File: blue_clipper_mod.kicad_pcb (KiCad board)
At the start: 2 copper layers, 68.6 x 50.8 mm, 23 parts, among them J1 AudioJack3, J2 AudioJack2, SW1 SW_Rotary_1x4_MP, SW2 SW_Rotary_1x4_MP, U1 RC4558

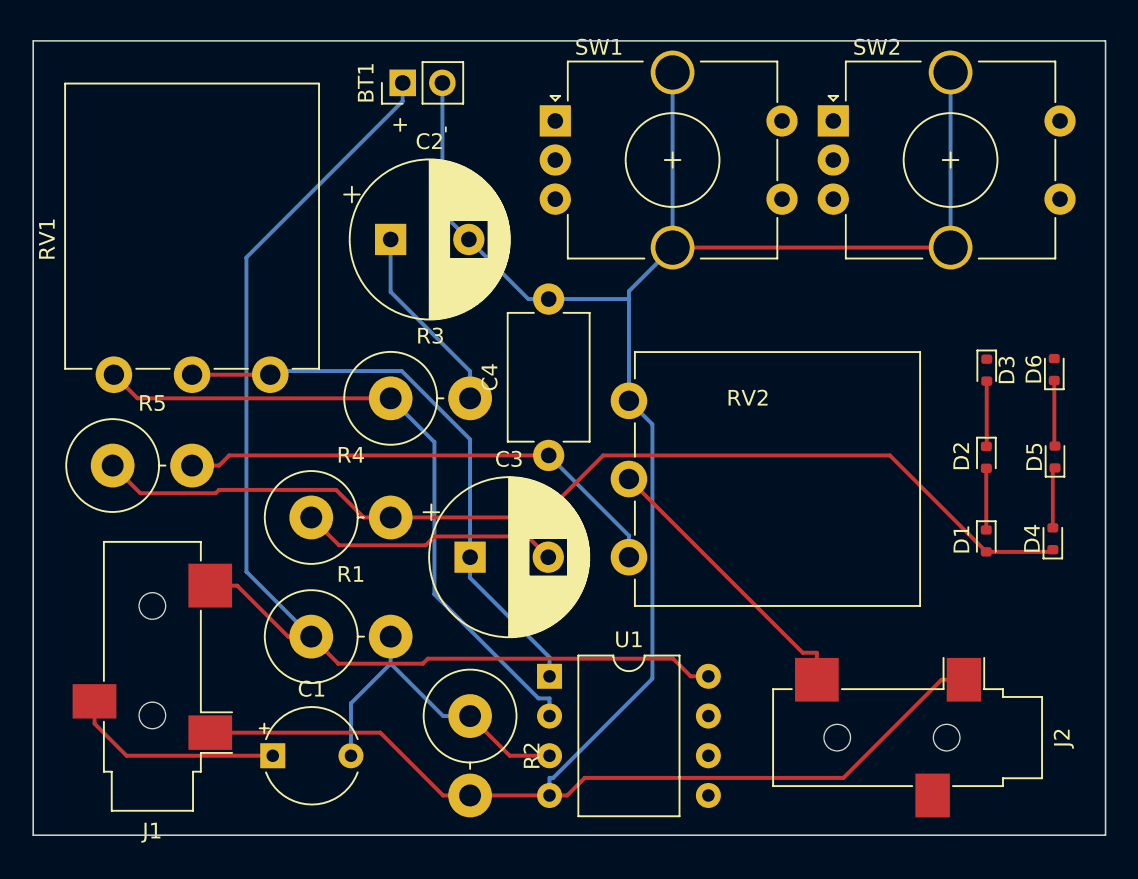
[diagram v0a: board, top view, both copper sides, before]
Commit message: Revert "reran autoroute"
This reverts commit 381ba4100bb96fee684d495079d12acf929bcbfa.
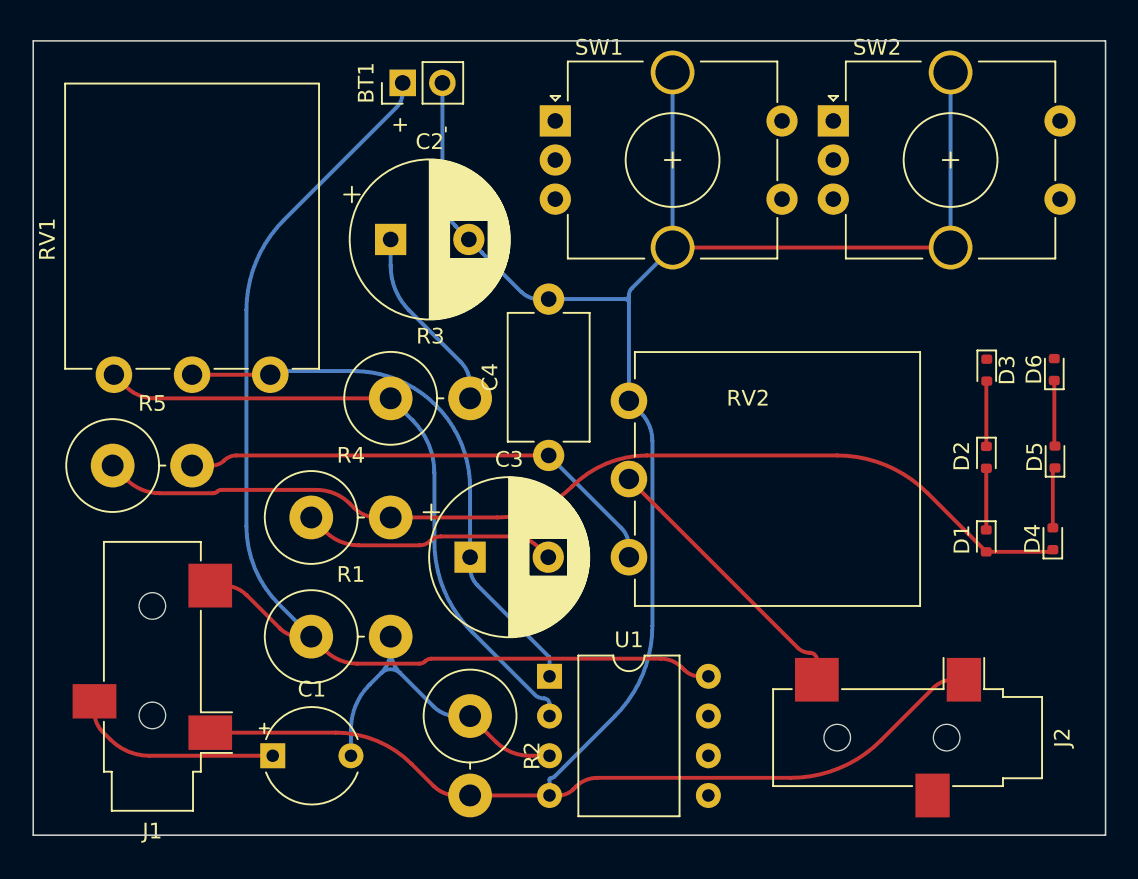
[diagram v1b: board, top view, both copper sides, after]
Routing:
- net Net-(U1A-+): track 21.3 -> 22.8 mm
- net /CLIPPER: track 65.9 -> 64.5 mm
- net GND: track 155.3 -> 154.0 mm
- net +9V: track 75.8 -> 74.5 mm
- net Net-(U1A--): track 43.3 -> 42.3 mm
- net Net-(C3-Pad1): track 36.9 -> 36.1 mm

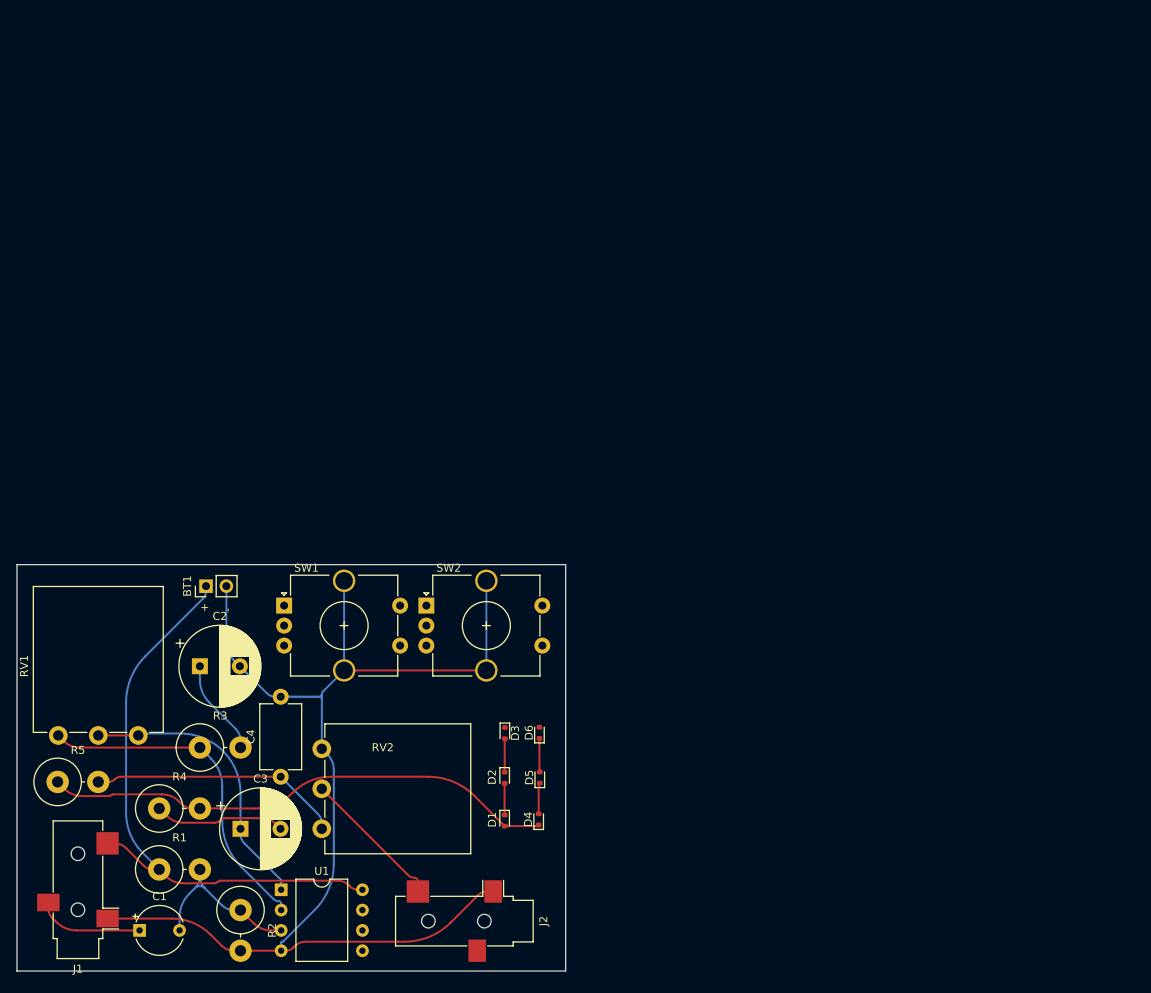
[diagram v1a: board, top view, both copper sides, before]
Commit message: fix everything
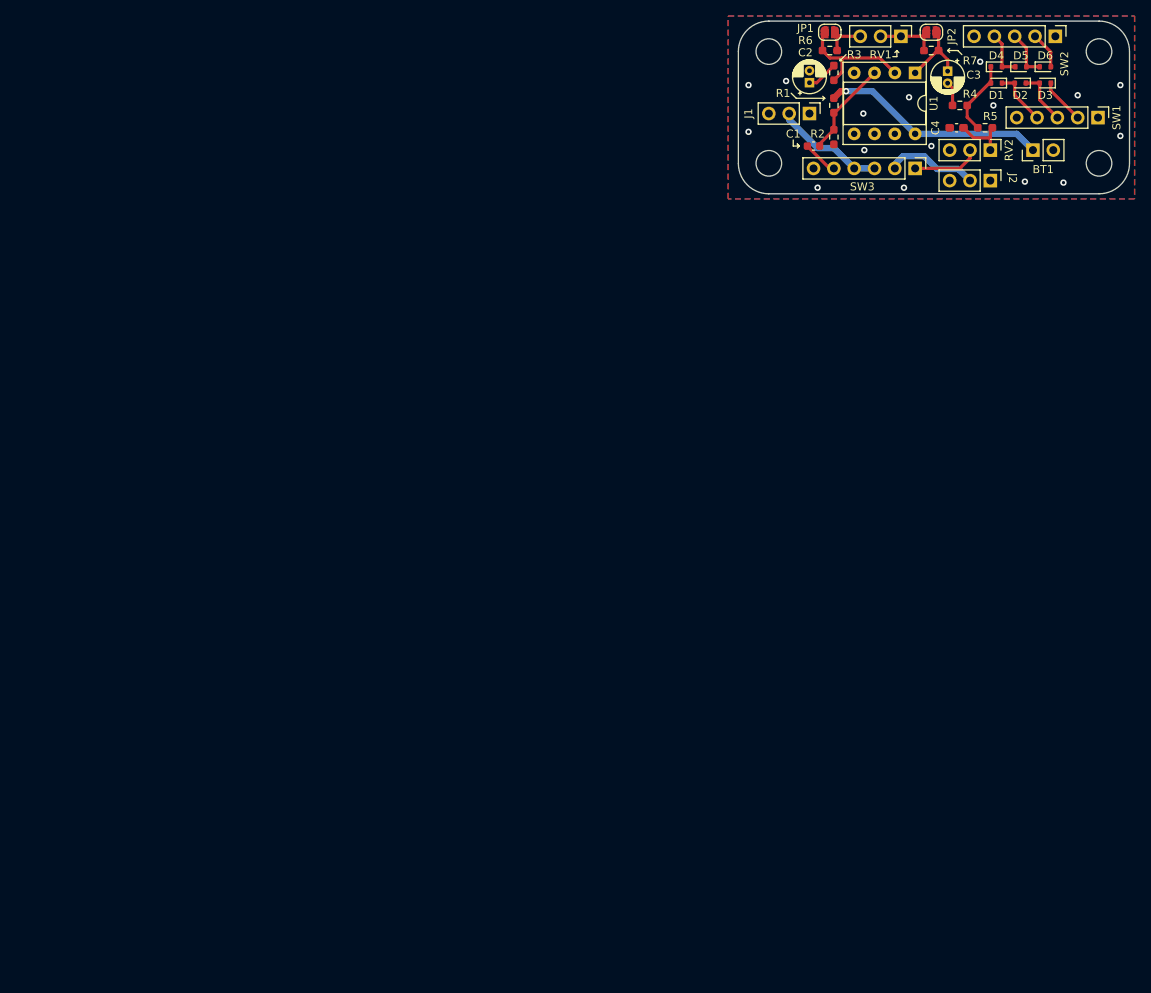
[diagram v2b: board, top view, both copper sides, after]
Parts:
- added H1: MountingHole, MountingHole:MountingHole_3.2mm_M3, F.Cu at (178.4, 50.2)
- added H2: MountingHole, MountingHole:MountingHole_3.2mm_M3, F.Cu at (137.2, 50.2)
- added H3: MountingHole, MountingHole:MountingHole_3.2mm_M3, F.Cu at (178.4, 64.1)
- added H4: MountingHole, MountingHole:MountingHole_3.2mm_M3, F.Cu at (137.2, 64.1)
- added JP1: SolderJumper_2_Open, Jumper:SolderJumper-2_P1.3mm_Open_RoundedPad1.0x1.5mm, F.Cu at (144.8, 47.8)
- added JP2: SolderJumper_2_Open, Jumper:SolderJumper-2_P1.3mm_Open_RoundedPad1.0x1.5mm, F.Cu at (157.5, 47.8)
- added R6: 50k, Resistor_SMD:R_0603_1608Metric_Pad0.98x0.95mm_HandSolder, F.Cu at (144.8, 50.0)
- added R7: 50k, Resistor_SMD:R_0603_1608Metric_Pad0.98x0.95mm_HandSolder, F.Cu at (157.5, 50.0)
- added SW3: BYPASS, Connector_PinHeader_2.54mm:PinHeader_1x06_P2.54mm_Vertical, F.Cu at (155.4, 64.8)
- C1: footprint Capacitor_THT:CP_Radial_Tantal_D6.0mm_P5.00mm -> Capacitor_SMD:C_0603_1608Metric
- C2, C3: footprint Capacitor_THT:CP_Radial_D10.0mm_P5.00mm -> Capacitor_THT:CP_Radial_D4.0mm_P1.50mm
- C4: footprint Capacitor_THT:C_Disc_D8.0mm_W5.0mm_P10.00mm -> Capacitor_SMD:C_0603_1608Metric_Pad1.08x0.95mm_HandSolder
- J1: value AudioJack3 -> IN; footprint Connector_Audio:Jack_3.5mm_CUI_SJ-3523-SMT_Horizontal -> custom:jack_pads
- J2: value AudioJack2 -> OUT; footprint Connector_Audio:Jack_3.5mm_CUI_SJ-3523-SMT_Horizontal -> custom:jack_pads
- R1, R3, R4, R5: footprint Resistor_THT:R_Axial_DIN0614_L14.3mm_D5.7mm_P5.08mm_Vertical -> Resistor_SMD:R_0603_1608Metric_Pad0.98x0.95mm_HandSolder
- R2: value 240k -> 20k; footprint Resistor_THT:R_Axial_DIN0614_L14.3mm_D5.7mm_P5.08mm_Vertical -> Resistor_SMD:R_0603_1608Metric_Pad0.98x0.95mm_HandSolder
- RV1: value 200k -> 100k; footprint Potentiometer_THT:Potentiometer_Piher_PC-16_Single_Vertical -> Connector_PinHeader_2.54mm:PinHeader_1x03_P2.54mm_Vertical
- RV2: footprint Potentiometer_THT:Potentiometer_Piher_PC-16_Single_Vertical -> Connector_PinHeader_2.54mm:PinHeader_1x03_P2.54mm_Vertical
- SW1, SW2: value SW_Rotary_1x4_MP -> ~; footprint Rotary_Encoder:RotaryEncoder_Alps_EC12E-Switch_Vertical_H20mm_CircularMountingHoles -> Connector_PinHeader_2.54mm:PinHeader_1x05_P2.54mm_Vertical
- U1: footprint Package_DIP:DIP-8_W10.16mm -> Package_DIP:DIP-8_W7.62mm_Socket
- moved R5 141.9 mm to (164.2, 59.7)
- moved R4 133.2 mm to (161.0, 56.9)
- moved J1 131.6 mm to (139.7, 57.9), turned to -90 degrees
- moved C3 129.5 mm to (159.5, 52.6), turned to -90 degrees
- moved RV1 129.3 mm to (153.7, 48.3), turned to -90 degrees
- moved C1 129.3 mm to (142.7, 62.0)
- moved U1 129.3 mm to (155.4, 52.8), turned to -90 degrees
- moved R1 127.4 mm to (145.3, 56.9), turned to -90 degrees
- moved R2 121.8 mm to (145.3, 60.9)
- moved RV2 119.1 mm to (164.8, 62.5), turned to -90 degrees
- moved SW1 118.6 mm to (178.3, 58.4), turned to -90 degrees
- moved C4 117.1 mm to (160.6, 59.7), turned to 180 degrees
- moved BT1 116.9 mm to (170.2, 62.5)
- moved R3 115.7 mm to (145.3, 52.8), turned to 90 degrees
- moved J2 112.1 mm to (162.3, 66.3)
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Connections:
- C1 pad 1: Net-(C1-Pad1) -> /EFFECT_IN
- C3 pad 1: Net-(C3-Pad1) -> Net-(JP2-B)
- J1 pad T: +9V -> /IN
- J2 pad T: Net-(J2-PadT) -> /OUT
- R3 pad 1: Net-(U1A--) -> Net-(JP1-A)
- RV1 pad 1: Net-(C3-Pad1) -> Net-(JP2-A)
- RV1 pad 2: Net-(C3-Pad1) -> Net-(JP2-A)
- RV1 pad 3: Net-(U1A--) -> Net-(JP1-B)
- RV2 pad 2: Net-(J2-PadT) -> /EFFECT_OUT
- U1 pad 1: Net-(C3-Pad1) -> Net-(JP2-B)
- U1 pad 2: Net-(U1A--) -> Net-(JP1-A)
- U1 pad 5: (no net) -> GND
- U1 pad 6: (no net) -> GND
- U1 pad 7: (no net) -> unconnected-(U1-Pad7)
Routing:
- net GND: track 154.0 -> 0.00 mm, vias 0 -> 16
- net /CLIPPER: track 64.5 -> 9.50 mm
- net +9V: track 74.5 -> 28.3 mm, vias 0 -> 1
- net Net-(U1A--): track 42.3 -> 0.00 mm
- net Net-(C3-Pad1): track 36.1 -> 0.00 mm
- net Net-(C4-Pad1): track 31.5 -> 6.78 mm
- net Net-(J2-PadT): track 18.1 -> 0.00 mm
- net Net-(JP1-A): track 0.00 -> 15.8 mm
- net /IN: track 0.00 -> 14.0 mm
- net Net-(C1-Pad1): track 13.4 -> 0.00 mm
- net Net-(C3-Pad2): track 16.3 -> 3.03 mm
- net /OUT: track 0.00 -> 11.6 mm
- net Net-(U1A-+): track 22.8 -> 12.0 mm
- net Net-(JP2-B): track 0.00 -> 9.52 mm
- net /EFFECT_OUT: track 0.00 -> 8.40 mm
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- added copper zone on B.Cu, net GND
- added copper zone on F.Cu, net GND
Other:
- board size 68.6 x 50.8 mm -> 48.9 x 21.6 mm
